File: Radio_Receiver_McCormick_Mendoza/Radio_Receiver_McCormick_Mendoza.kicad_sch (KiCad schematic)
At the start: 1 part, among them U1 RP2040

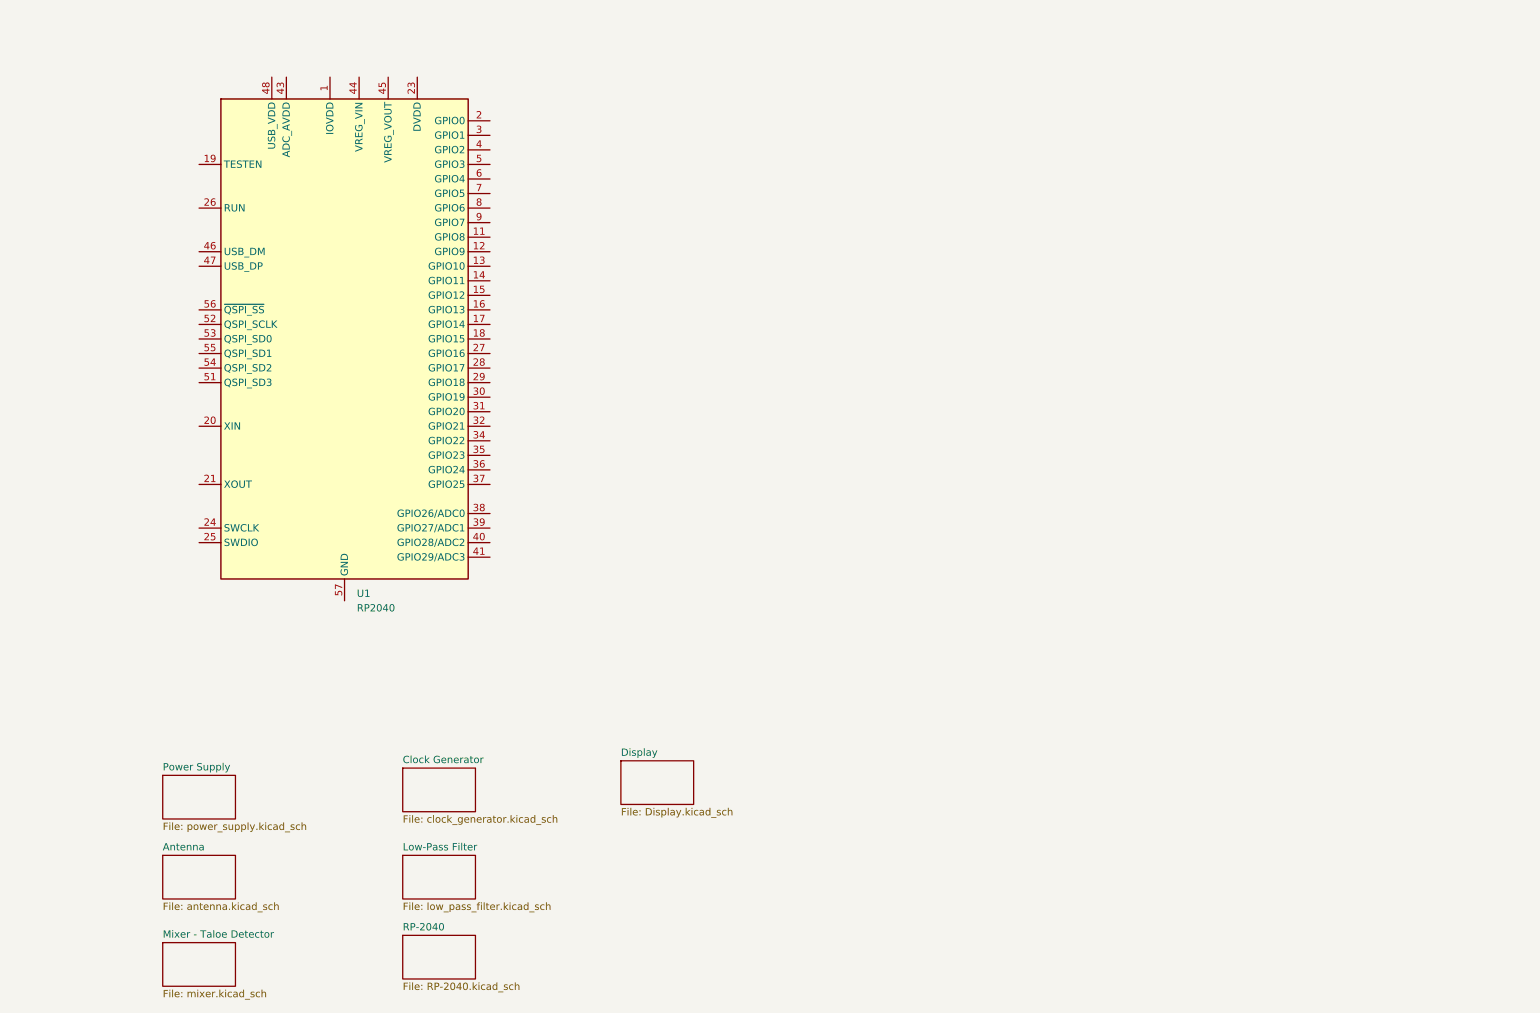
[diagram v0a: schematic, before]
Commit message: Added Bibliography entry
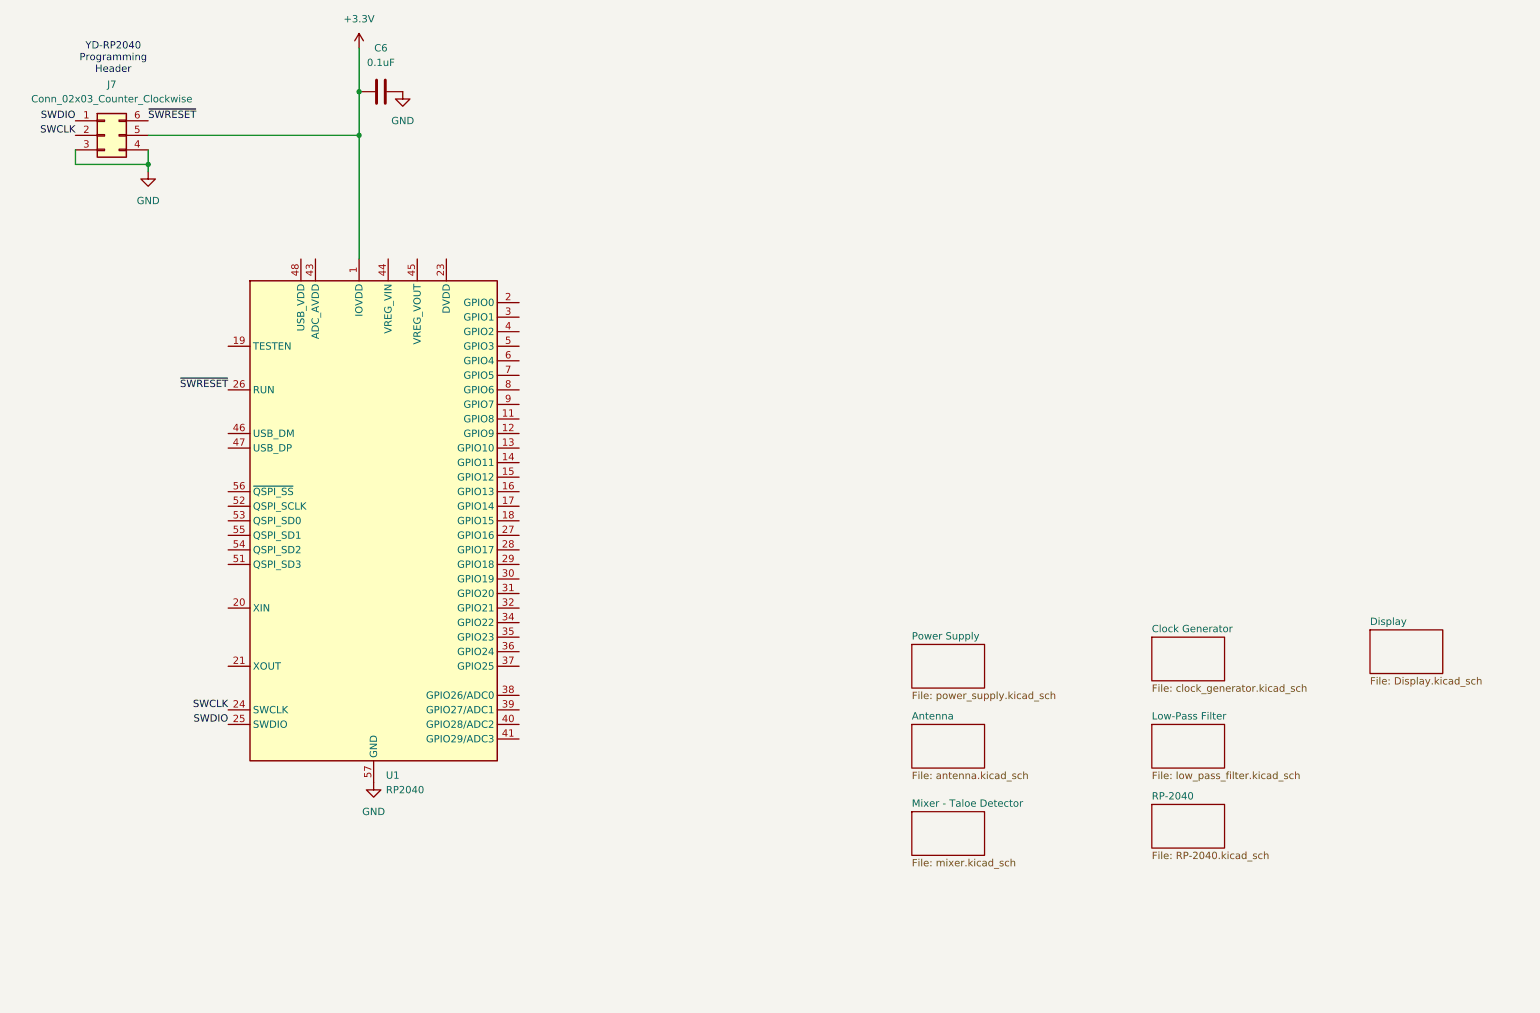
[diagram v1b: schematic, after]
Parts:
- added C6: 0.1uF, symbol Device:C
- added J7: Conn_02x03_Counter_Clockwise, symbol Connector_Generic:Conn_02x03_Counter_Clockwise
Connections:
- net +3.3V: now reaches U1.1 (IOVDD), U1.10 (IOVDD), U1.22 (IOVDD), U1.33 (IOVDD), U1.42 (IOVDD), U1.49 (IOVDD)
- net +3.3V: now also C6.1, J7.5 (Pin_5)
- net SWCLK: now reaches U1.24 (SWCLK)
- net SWCLK: now also J7.2 (Pin_2)
- net SWDIO: now reaches U1.25 (SWDIO)
- net SWDIO: now also J7.1 (Pin_1)
- net ~{SWRESET}: now reaches U1.26 (RUN)
- net ~{SWRESET}: now also J7.6 (Pin_6)
- net GND: now reaches U1.57 (GND)
- net GND: now also C6.2, J7.3 (Pin_3), J7.4 (Pin_4)
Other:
- note added: "YD-RP2040 Programming Header"
- moved on the sheet: U1
